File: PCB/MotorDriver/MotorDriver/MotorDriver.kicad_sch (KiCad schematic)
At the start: 1 part, among them J3 XT30PW-M

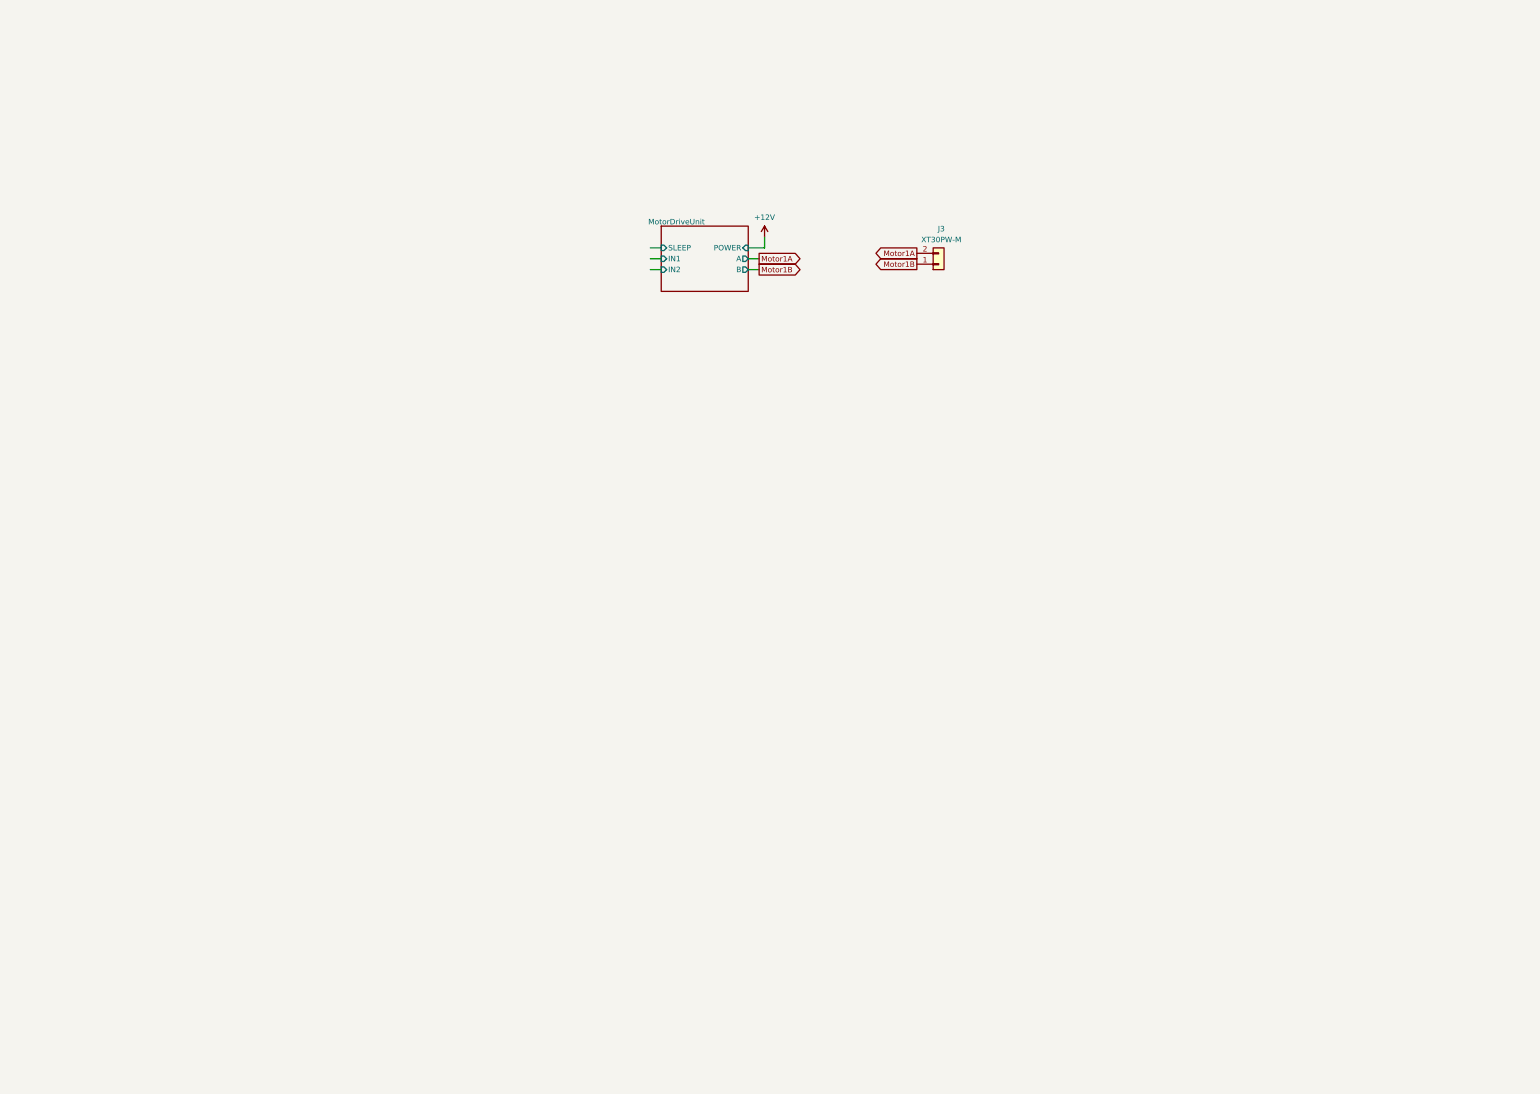
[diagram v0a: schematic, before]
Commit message: :sparkles: 基板V2完成！！！
MotorDriverになってるけど普通にMain PCB V2ですわ！
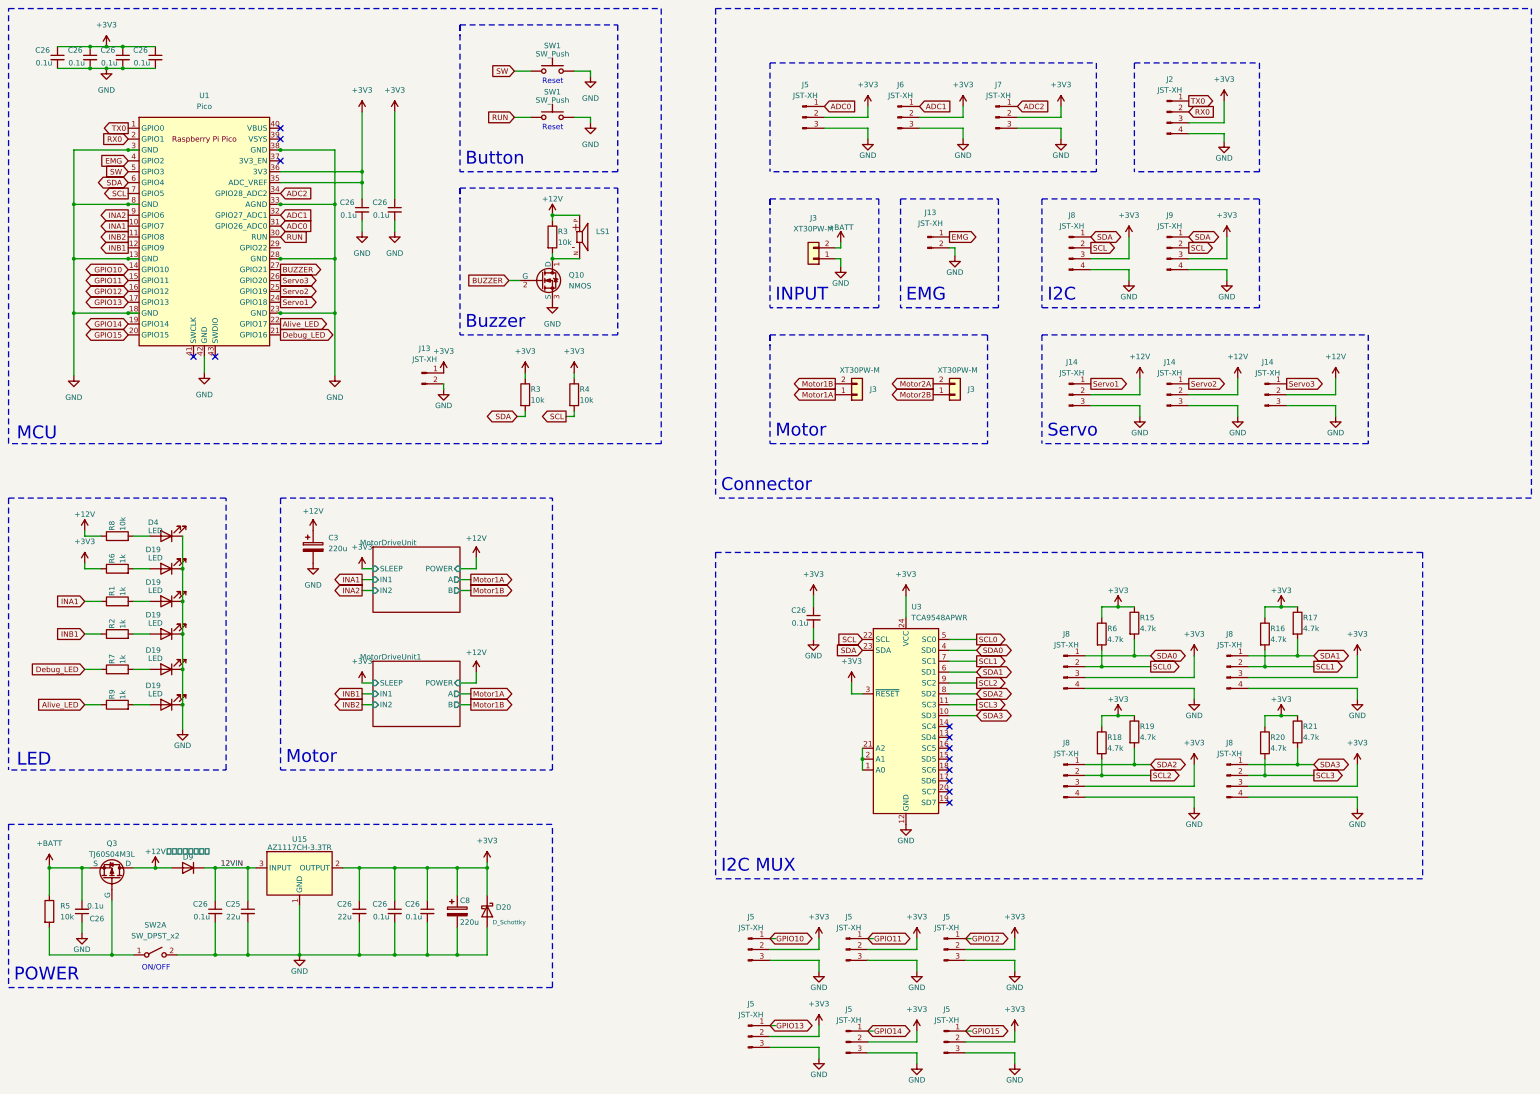
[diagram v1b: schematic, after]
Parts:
- removed J3: XT30PW-M, Connector_AMASS:AMASS_XT30PW-M_1x02_P2.50mm_Horizontal, symbol Connector_Generic:Conn_01x02
- added C25, C26: 22u, Capacitor_SMD:C_1206_3216Metric_Pad1.33x1.80mm_HandSolder, symbol Device:C_Small
- added C26 (x11): 0.1u, Capacitor_SMD:C_0603_1608Metric_Pad1.08x0.95mm_HandSolder, symbol Device:C_Small
- added C3: 220u, Capacitor_SMD:CP_Elec_10x10, symbol Device:C_Polarized
- added C8: 220u, Capacitor_SMD:CP_Elec_6.3x5.4, symbol Device:C_Polarized
- added D19 (x5), D4: LED, LED_SMD:LED_0603_1608Metric_Pad1.05x0.95mm_HandSolder, symbol Device:LED
- added D20: D_Schottky, Diode_SMD:D_SOD-323_HandSoldering, symbol Device:D_Schottky
- added D9: ＧＳ１０１０ＦＬ, Diode_SMD:D_SOD-123F, symbol Device:D
- added J13 (x2): JST-XH, Connector_JST:JST_XH_B2B-XH-A_1x02_P2.50mm_Vertical, symbol Connector:Conn_01x02_Pin
- added J14 (x3), J5, J6, J7: JST-XH, Connector_JST:JST_XH_B3B-XH-A_1x03_P2.50mm_Vertical, symbol Connector:Conn_01x03_Pin
- added J2, J8 (x5), J9: JST-XH, Connector_JST:JST_XH_B4B-XH-A_1x04_P2.50mm_Vertical, symbol Connector:Conn_01x04_Pin
- added J3 (x3): XT30PW-M, Connector_AMASS:AMASS_XT30PW-M_1x02_P2.50mm_Horizontal, symbol Connector_Generic:Conn_01x02
- added J5 (x6): JST-XH, Connector_PinHeader_2.54mm:PinHeader_1x03_P2.54mm_Vertical, symbol Connector:Conn_01x03_Pin
- added LS1: PKLCS1212E4001-R1, PKLCS1212E4001-R1:PKL, symbol PKLCS1212E4001-R1:PKLCS1212E4001-R1
- added Q10: NMOS, Package_TO_SOT_SMD:SOT-23, symbol Simulation_SPICE:NMOS
- added Q3: TJ60S04M3L, Package_TO_SOT_SMD:TO-252-2, symbol Simulation_SPICE:PMOS
- added R1, R2, R6, R7, R9: 1k, Resistor_SMD:R_0603_1608Metric_Pad0.98x0.95mm_HandSolder, symbol Device:R
- added R15, R16, R17, R18, R19, R20, R21, R6: 4.7k, Resistor_SMD:R_0402_1005Metric_Pad0.72x0.64mm_HandSolder, symbol Device:R
- added R3 (x2), R4, R5, R8: 10k, Resistor_SMD:R_0603_1608Metric_Pad0.98x0.95mm_HandSolder, symbol Device:R
- added SW1 (x2): SW_Push, newinov-kicad:SKRPACE010, symbol Switch:SW_Push
- added SW2: SW_DPST_x2, Button_Switch_THT:SW_E-Switch_EG1271_SPDT, symbol Switch:SW_DPST_x2
- added U1: Pico, MCU_RaspberryPi_and_Boards:RPi_Pico_SMD_TH, symbol MCU_RaspberryPi_and_Boards:Pico
- added U15: AZ1117CH-3.3TR, Package_TO_SOT_SMD:SOT-223-3_TabPin2, symbol sushi_lib:AZ1117CH-3.3TR
- added U3: TCA9548APWR, Package_SO:TSSOP-24_4.4x7.8mm_P0.65mm, symbol Interface_Expansion:TCA9548APWR
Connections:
- net +12V: now also C3.1, D9.2 (A), J14.2 (Pin_2), J14.2 (Pin_2), J14.2 (Pin_2), LS1.P, Q3.2 (D), R3.1, R8.1
- net Motor1A: now also J3.1 (Pin_1)
- net Motor1B: now also J3.2 (Pin_2)
- new net: D19.2 (A), R2.2
- new net: U3.1 (A0), U3.2 (A1), U3.21 (A2)
- new net: D4.2 (A), R8.2
- new net: D19.2 (A), R1.2
- new net: D19.2 (A), R6.2
- new net: D19.2 (A), R7.2
- new net: LS1.N, Q10.1 (D), R3.2
- new net: D19.2 (A), R9.2
- new net: Q3.1 (G), R5.2, SW2.1 (A)
- new net +3V3: C26.1, C26.1, C26.1, C26.1, C26.1, C26.1, C26.1, C26.1, C26.1, C26.1, C8.1, D20.1 (K), J13.1 (Pin_1), J2.3 (Pin_3), J5.2 (Pin_2), J5.2 (Pin_2), J5.2 (Pin_2), J5.2 (Pin_2), J5.2 (Pin_2), J5.2 (Pin_2), J5.2 (Pin_2), J6.2 (Pin_2), J7.2 (Pin_2), J8.3 (Pin_3), J8.3 (Pin_3), J8.3 (Pin_3), J8.3 (Pin_3), J8.3 (Pin_3), J9.3 (Pin_3), R15.1, R16.1, R17.1, R18.1, R19.1, R20.1, R21.1, R3.1, R4.1, R6.1, R6.1, U1.35 (ADC_VREF), U1.36 (3V3), U15.2 (OUTPUT), U3.24 (VCC), U3.3 (~{RESET})
- new net +BATT: C26.2, J3.2 (Pin_2), Q3.3 (S), R5.1
- new net 12VIN: C25.1, C26.1, D9.1 (K), U15.3 (INPUT)
- new net ADC0: J5.1 (Pin_1), U1.31 (GPIO26_ADC0)
- new net ADC1: J6.1 (Pin_1), U1.32 (GPIO27_ADC1)
- new net ADC2: J7.1 (Pin_1), U1.34 (GPIO28_ADC2)
- new net Alive_LED: R9.1, U1.22 (GPIO17)
- new net BUZZER: Q10.2 (G), U1.27 (GPIO21)
- new net Debug_LED: R7.1, U1.21 (GPIO16)
- new net EMG: J13.1 (Pin_1), U1.4 (GPIO2)
- new net GND: C25.2, C26.1, C26.2, C26.2, C26.2, C26.2, C26.2, C26.2, C26.2, C26.2, C26.2, C26.2, C26.2, C3.2, C8.2, D19.1 (K), D19.1 (K), D19.1 (K), D19.1 (K), D19.1 (K), D20.2 (A), D4.1 (K), J13.2 (Pin_2), J13.2 (Pin_2), J14.3 (Pin_3), J14.3 (Pin_3), J14.3 (Pin_3), J2.4 (Pin_4), J3.1 (Pin_1), J5.3 (Pin_3), J5.3 (Pin_3), J5.3 (Pin_3), J5.3 (Pin_3), J5.3 (Pin_3), J5.3 (Pin_3), J5.3 (Pin_3), J6.3 (Pin_3), J7.3 (Pin_3), J8.4 (Pin_4), J8.4 (Pin_4), J8.4 (Pin_4), J8.4 (Pin_4), J8.4 (Pin_4), J9.4 (Pin_4), Q10.3 (S), SW1.1, SW1.1, SW2.2 (B), U1.13 (GND), U1.18 (GND), U1.23 (GND), U1.28 (GND), U1.3 (GND), U1.33 (AGND), U1.38 (GND), U1.42 (GND), U1.8 (GND), U15.1 (GND), U3.12 (GND)
- new net GPIO10: J5.1 (Pin_1), U1.14 (GPIO10)
- new net GPIO11: J5.1 (Pin_1), U1.15 (GPIO11)
- new net GPIO12: J5.1 (Pin_1), U1.16 (GPIO12)
- new net GPIO13: J5.1 (Pin_1), U1.17 (GPIO13)
- new net GPIO14: J5.1 (Pin_1), U1.19 (GPIO14)
- new net GPIO15: J5.1 (Pin_1), U1.20 (GPIO15)
- new net INA1: R1.1, U1.10 (GPIO7)
- new net INA2: U1.9 (GPIO6)
- new net INB1: R2.1, U1.12 (GPIO9)
- new net INB2: U1.11 (GPIO8)
- new net Motor2A: J3.2 (Pin_2)
- new net Motor2B: J3.1 (Pin_1)
- new net RUN: SW1.2, U1.30 (RUN)
- new net RX0: J2.2 (Pin_2), U1.2 (GPIO1)
- new net SCL: J8.2 (Pin_2), J9.2 (Pin_2), R4.2, U1.7 (GPIO5), U3.22 (SCL)
- new net SCL0: J8.2 (Pin_2), R6.2, U3.5 (SC0)
- new net SCL1: J8.2 (Pin_2), R16.2, U3.7 (SC1)
- new net SCL2: J8.2 (Pin_2), R18.2, U3.9 (SC2)
- new net SCL3: J8.2 (Pin_2), R20.2, U3.11 (SC3)
- new net SDA: J8.1 (Pin_1), J9.1 (Pin_1), R3.2, U1.6 (GPIO4), U3.23 (SDA)
- new net SDA0: J8.1 (Pin_1), R15.2, U3.4 (SD0)
- new net SDA1: J8.1 (Pin_1), R17.2, U3.6 (SD1)
- new net SDA2: J8.1 (Pin_1), R19.2, U3.8 (SD2)
- new net SDA3: J8.1 (Pin_1), R21.2, U3.10 (SD3)
- new net SW: SW1.2, U1.5 (GPIO3)
- new net Servo1: J14.1 (Pin_1), U1.24 (GPIO18)
- new net Servo2: J14.1 (Pin_1), U1.25 (GPIO19)
- new net Servo3: J14.1 (Pin_1), U1.26 (GPIO20)
- new net TX0: J2.1 (Pin_1), U1.1 (GPIO0)
- no-connect marks 0 -> 13
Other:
- added sheet MotorDriveUnit1 (H-Bridge.kicad_sch)
- note added: "Button"
- note added: "Buzzer"
- note added: "Connector"
- note added: "EMG"
- note added: "I2C"
- note added: "I2C MUX"
- note added: "INPUT"
- note added: "LED"
- note added: "MCU"
- note added: "Motor"
- note added: "ON/OFF"
- note added: "POWER"
- note added: "Reset"
- note added: "Servo"
